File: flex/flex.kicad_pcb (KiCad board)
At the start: 2 copper layers, 127 x 94.5 mm, 11 parts, among them J7 Conn_01x07_Socket, SW5 SW_Push, SW6 SW_Push, SW7 SW_Push, SW8 SW_Push

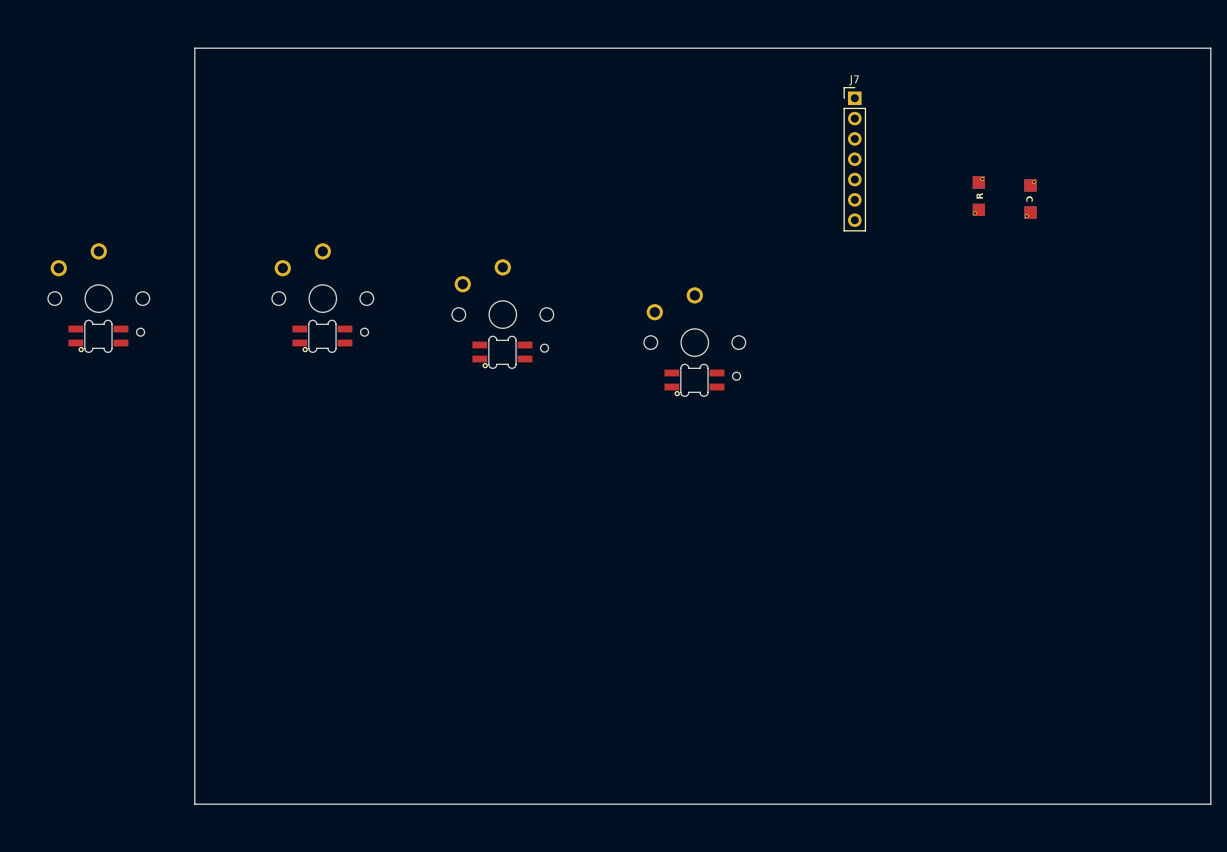
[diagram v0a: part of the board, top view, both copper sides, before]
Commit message: flex PCB
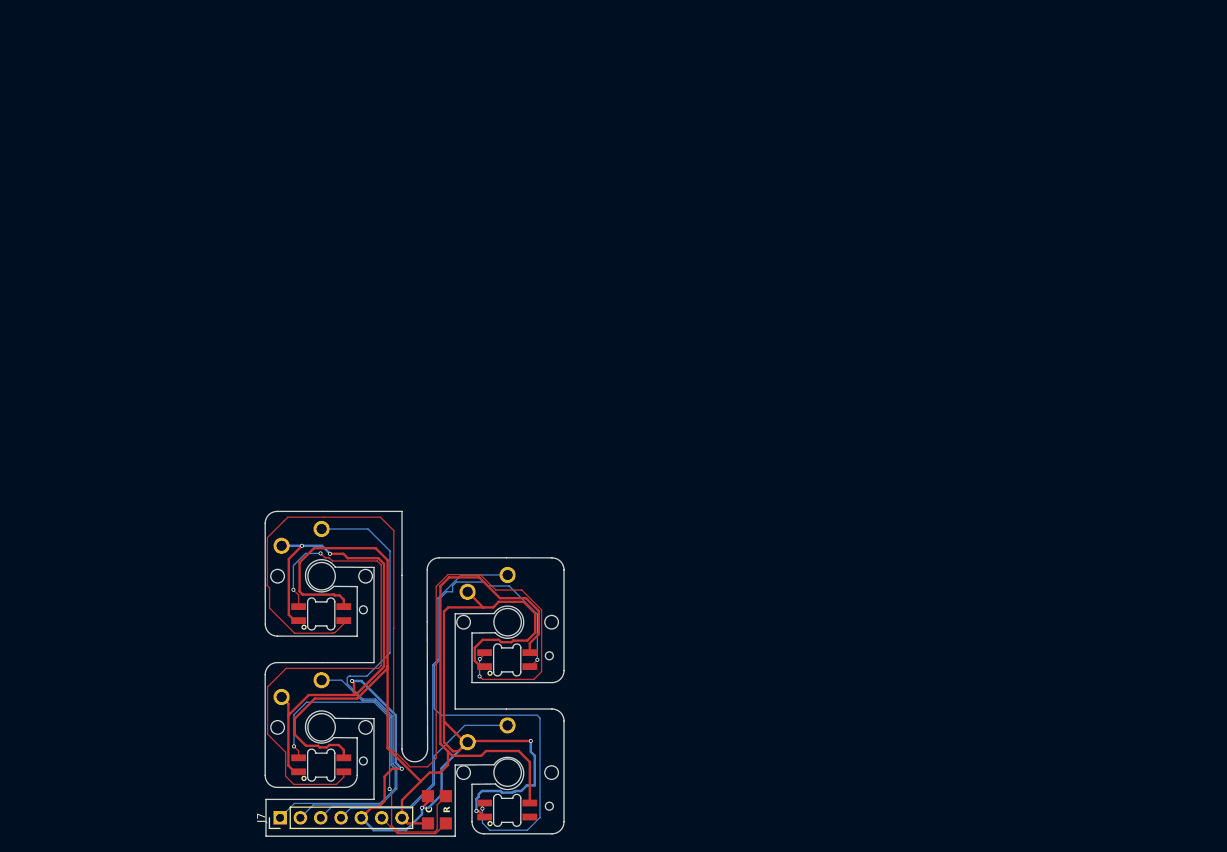
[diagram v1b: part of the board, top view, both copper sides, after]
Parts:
- moved J7 115.1 mm to (-97.3, 130.7), turned to 90 degrees
- moved C3 114.6 mm to (-78.8, 134.7), turned to 90 degrees
- moved R3 101.6 mm to (-76.6, 134.7)
- moved SW7 58.6 mm to (-68.9, 125.0)
- moved D16 58.6 mm to (-68.9, 129.6)
- moved SW6 53.6 mm to (-92.2, 119.4)
- moved D13 53.6 mm to (-92.2, 124.0)
- moved SW5 44.5 mm to (-92.2, 100.5)
- moved D14 44.5 mm to (-92.2, 105.1)
- moved SW8 38.5 mm to (-68.9, 106.2)
- moved D15 38.5 mm to (-68.9, 110.8)
- renumbered D14 to D13, D13 to D14
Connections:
- D13 pad 1: Net-(D14-DOUT) -> Net-(D13-DOUT)
- D13 pad 3: Net-(D13-DOUT) -> Net-(D13-DIN)
- D14 pad 1: Net-(D13-DOUT) -> Net-(D14-DOUT)
- D14 pad 3: Net-(D13-DIN) -> Net-(D13-DOUT)
- SW5 pad 1: sw1 -> sw2
- SW6 pad 1: sw3 -> sw1
- SW7 pad 1: sw2 -> sw4
- SW8 pad 1: sw4 -> sw3
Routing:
- net Gnd: track 0.00 -> 189.1 mm, vias 0 -> 7
- net Vcc: track 0.00 -> 149.4 mm
- net Net-(D14-DOUT): track 0.00 -> 128.4 mm, vias 0 -> 2
- net Net-(D15-DOUT): track 0.00 -> 73.1 mm, vias 0 -> 2
- net Net-(D13-DOUT): track 0.00 -> 66.3 mm, vias 0 -> 2
- net sw2: track 0.00 -> 60.1 mm
- net sw3: track 0.00 -> 49.2 mm
- net Net-(D13-DIN): track 0.00 -> 43.4 mm, vias 0 -> 2
- net sw1: track 0.00 -> 35.6 mm
- net sw4: track 0.00 -> 27.7 mm
- net Din: track 0.00 -> 9.36 mm
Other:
- board size 127 x 94.5 mm -> 37.4 x 40.6 mm
